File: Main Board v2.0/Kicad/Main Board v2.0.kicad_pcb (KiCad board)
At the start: 4 copper layers, 172.7 x 83.9 mm, 81 parts, among them J1 Bus_ISA_16bit, J2 +3V3 Supply, J3 JTAG, J4 AVR-JTAG-10, J5 USART0, J6 USART1, J7 PS2KB, J8 SPI-SDCard, SW1 Reset, U1 74HCT245, U10 74HCT245, U11 ATmega1284-P, U2 GLT725608, U3 74HCT245, U4 GLT725608, U5 AS6C4008-55PCN, U6 AM29F040B, U7 XC95288XL-TQ144, U8 AP1117-33, U9 Z80CPU, Y1 20MHz, Y2 32.768kHz

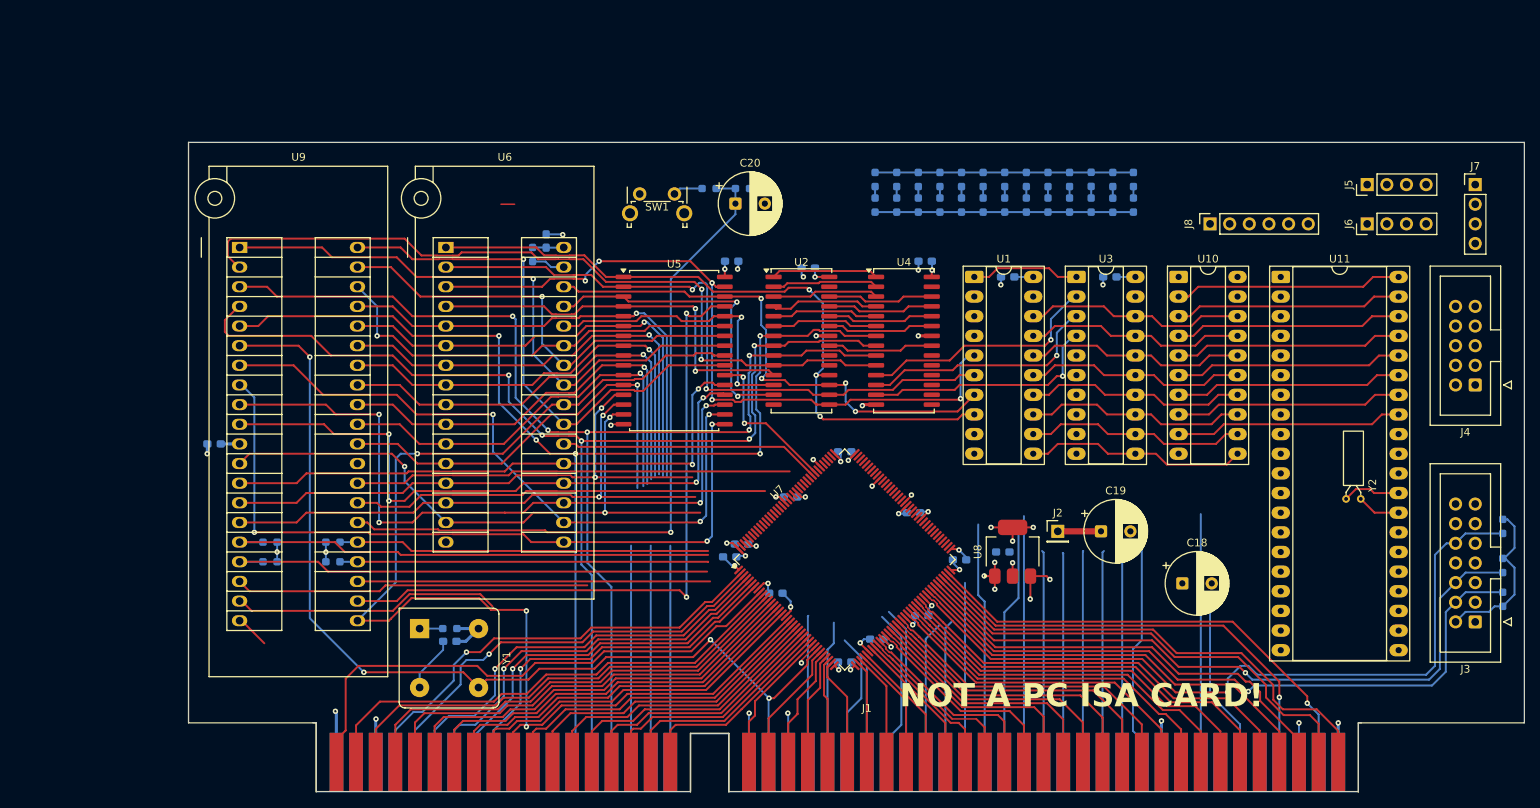
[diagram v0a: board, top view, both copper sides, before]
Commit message: board progress
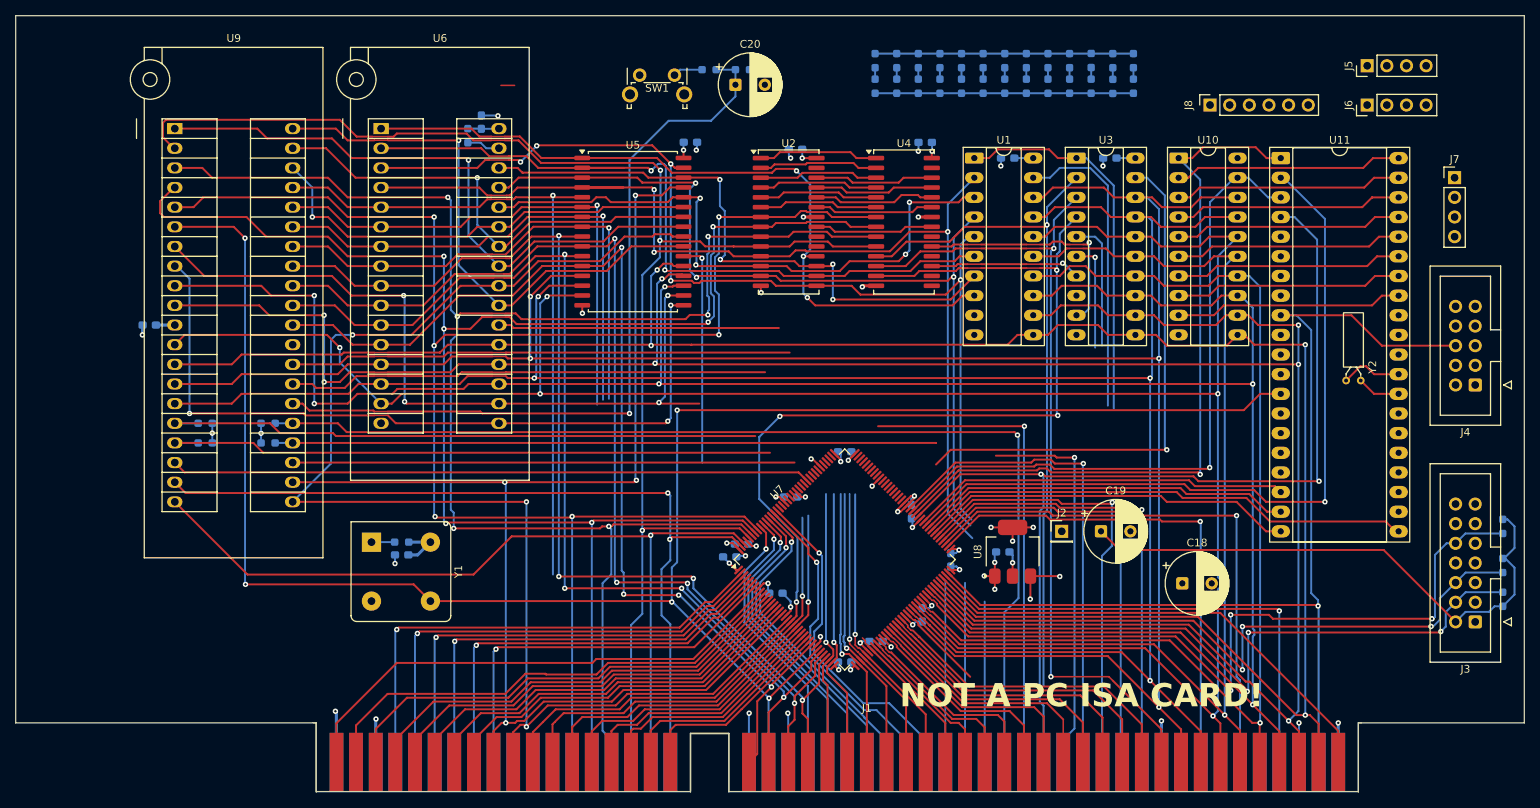
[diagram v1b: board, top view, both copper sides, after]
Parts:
- U1, U10, U3: footprint Package_DIP:DIP-20_W7.62mm_Socket_LongPads -> Library:DIP-20_W7.62mm_Socket_LongNarrowPads
- moved C21 17.5 mm to (91.5, 87.0)
- moved C6 17.5 mm to (134.4, 60.7)
- moved R27 17.5 mm to (132.7, 62.5)
- moved R39 17.5 mm to (98.7, 99.7)
- moved R40 17.5 mm to (106.9, 99.7)
- moved U6 17.5 mm to (121.5, 61.6)
- moved U9 17.5 mm to (94.8, 61.6)
- moved R36 17.5 mm to (106.9, 102.2)
- moved R38 17.5 mm to (98.7, 102.2)
- moved U5 16.3 mm to (154.0, 74.9)
- moved C5 16.3 mm to (161.5, 63.3)
- moved U2 15.5 mm to (174.2, 73.6)
- moved C2 15.5 mm to (175.1, 64.2)
- moved R1 15.4 mm to (216.1, 52.8)
- moved R10 15.4 mm to (202.1, 52.8)
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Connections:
- U7 pad 120: SYSDDIR -> ~{CPU_INT}
- U7 pad 121: ~{SYSDEN} -> ~{BIACK}
- U7 pad 124: SYSCMD -> ~{CPU_RFSH}
- U7 pad 125: SYSINTACK -> ~{CPU_BUSRQ}
- U7 pad 126: SYSINT0 -> BCLK
- U7 pad 128: SYSINT1 -> ~{CPU_BUSACK}
- U7 pad 129: SYSINT2 -> ~{CPU_NMI}
- U7 pad 130: ~{CPU_NMI} -> BINTACK1
- U7 pad 131: ~{CPU_INT} -> BINTACK2
- U7 pad 132: BINTACK1 -> BIRQ4
- U7 pad 133: BIRQ0 -> BIRQ3
- U7 pad 134: BIRQ1 -> BIRQ2
- U7 pad 135: BIRQ2 -> BIRQ1
- U7 pad 136: /CPU/A12 -> BIRQ0
- U7 pad 137: /CPU/A13 -> /CPU/A15
- U7 pad 139: /CPU/A15 -> /CPU/A13
- U7 pad 140: BIRQ3 -> A12
- U7 pad 74: ~{B8_MEM_WR} -> BINTACK4
- U7 pad 75: ~{B8_MEM_RD} -> BINTACK3
- U7 pad 76: ~{BIO_WR} -> ~{B8_MEM_WR}
- U7 pad 77: ~{BIO_RD} -> ~{B8_MEM_RD}
- U7 pad 78: ~{BIACK} -> ~{BIO_WR}
- U7 pad 79: BINTEN -> SYSINT2
- U7 pad 80: ~{CPU_BUSRQ} -> SYSINTACK
- U7 pad 81: ~{CPU_BUSACK} -> SYSINT1
- U7 pad 82: ~{CPU_RFSH} -> SYSCMD
- U7 pad 83: BCLK -> SYSINT0
- U7 pad 85: BINTACK2 -> BINTEN
- U7 pad 86: BINTACK3 -> SYSDDIR
- U7 pad 87: BINTACK4 -> ~{SYSDEN}
- U7 pad 88: BIRQ4 -> ~{BIO_RD}
- U9 pad 2: /CPU/A12 -> A12
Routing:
- net A12: track 0.00 -> 192.8 mm, vias 0 -> 3
- net /CPU/D6: track 171.1 -> 317.5 mm, vias 4 -> 7
- net /CPU/D2: track 158.6 -> 301.1 mm, vias 3 -> 5
- net /CPU/D0: track 147.2 -> 287.0 mm, vias 2 -> 4
- net /CPU/D5: track 175.8 -> 309.7 mm, vias 4 -> 6
- net /CPU/D1: track 150.9 -> 283.6 mm, vias 2 -> 4
- net /CPU/A12: track 129.0 -> 0.00 mm, vias 2 -> 0
- net CLK20: track 130.0 -> 250.1 mm, vias 4 -> 5
- net /CPU/D7: track 164.8 -> 274.1 mm, vias 2 -> 4
- net BINTEN: track 27.4 -> 129.7 mm, vias 0 -> 2
- net SYSCMD: track 0.00 -> 99.2 mm, vias 0 -> 1
- net SYSDDIR: track 0.00 -> 96.0 mm, vias 0 -> 1
- net /Control Logic/MA12: track 76.2 -> 163.4 mm, vias 2 -> 3
- net ~{SYSDEN}: track 0.00 -> 87.1 mm, vias 0 -> 1
- net /Control Logic/MA22: track 75.9 -> 161.5 mm, vias 1 -> 4
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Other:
- board size 172.7 x 83.9 mm -> 195.1 x 100.3 mm
